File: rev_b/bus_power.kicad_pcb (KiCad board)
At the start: 2 copper layers, 50 x 50 mm, 18 parts, among them J1 TERMINATE_JUMPER, Q1 FQP47P06, Q2 FQP47P06, SW1 F-426-0020

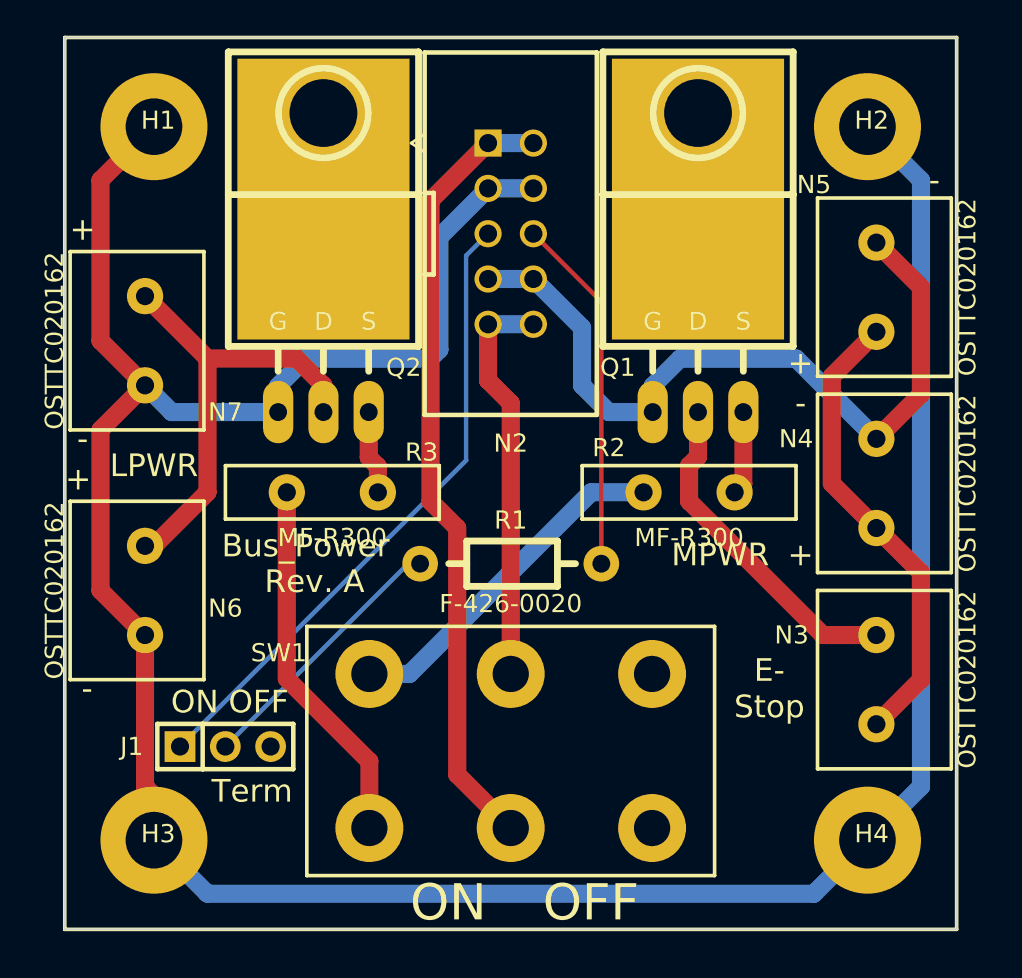
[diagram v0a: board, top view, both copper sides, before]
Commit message: Did first layout of Rev. B.
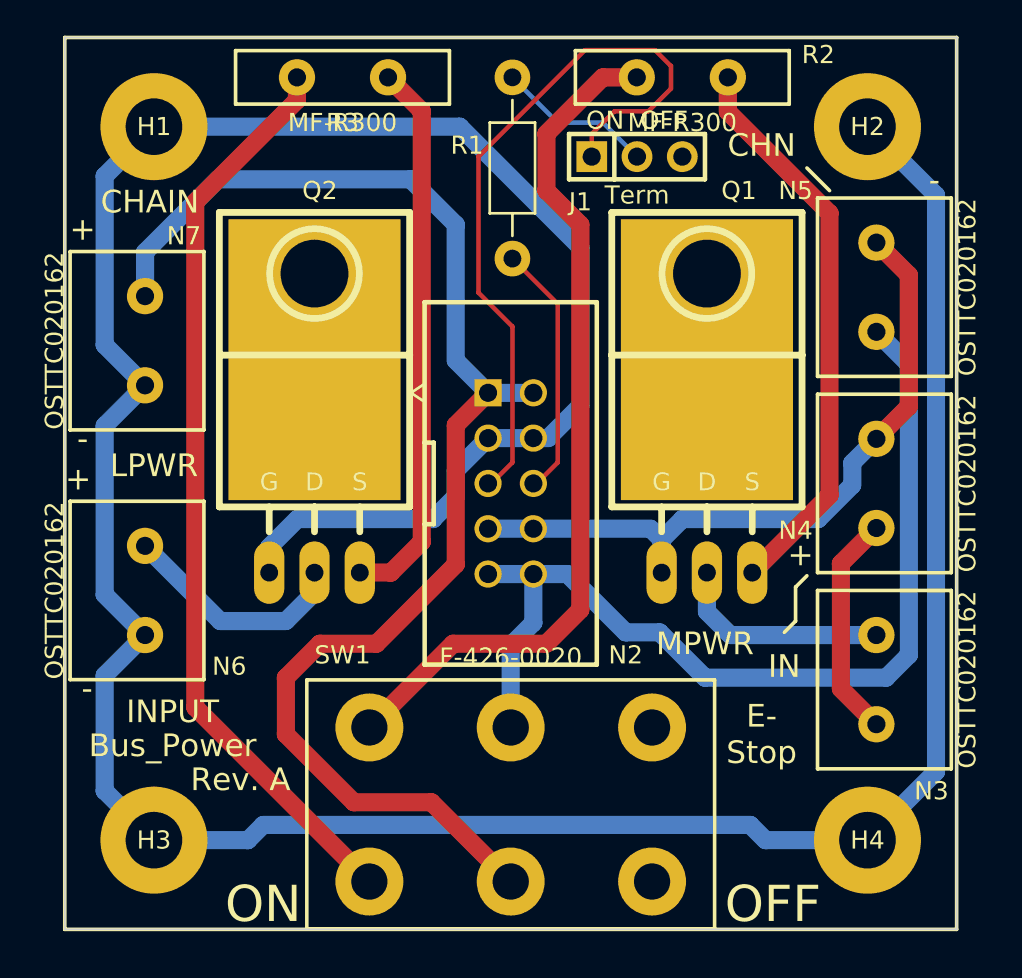
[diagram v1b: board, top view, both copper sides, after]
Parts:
- G1: footprint Bus_BeagleBone_Rev_A:OSHW_LOGO_400mil -> Bus_Power:OSHW_LOGO_400mil
- H1, H2, H3, H4: footprint Bus_BeagleBone_Rev_A:MountingHole_3mm -> Bus_Power:MountingHole_3mm
- J1: footprint Bus_BeagleBone_Rev_A:Pin_Header_Straight_1x03 -> Bus_Power:Pin_Header_Straight_1x03
- N2: footprint Bus_BeagleBone_Rev_A:Pin_Header_Straight_2x05_Shrouded -> Bus_Power:Pin_Header_Straight_2x05_Shrouded
- N3, N4, N5, N6, N7: footprint Bus_BeagleBone_Rev_A:5MM_TERMINAL_BLOCK_2_POS -> Bus_Power:5MM_TERMINAL_BLOCK_2_POS
- Q1, Q2: footprint Bus_BeagleBone_Rev_A:TO-220_FET-GDS_Horizontal_LargePads -> Bus_Power:TO-220_FET-GDS_Horizontal_LargePads
- R1: footprint Bus_BeagleBone_Rev_A:Resistor_Horizontal__400 -> Bus_Power:Resistor_Horizontal_400
- R2, R3: footprint Bus_Power_Rev_A:MF_R300 -> Bus_Power:MF_R300
- SW1: footprint Bus_Power_Rev_A:GF_426_0020 -> Bus_Power:GF_426_0020
- moved J1 40.3 mm to (132.1, 106.7)
- moved R3 23.3 mm to (115.6, 102.2)
- moved R2 23.3 mm to (134.6, 102.2)
- moved R1 22.2 mm to (125.1, 107.3), turned to 270 degrees
- moved N2 14.0 mm to (125.0, 125.0)
- moved G1 9.94 mm to (135.9, 120.0)
- moved Q1 9.01 mm to (136.0, 130.0)
- moved Q2 9.01 mm to (114.0, 130.0)
- moved SW1 3.00 mm to (125.0, 143.0)
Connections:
- net /BGND renamed /MGND
- net /BPWR2 renamed /MPWR1
- net /BPWR3 renamed /MPWR2
- net /BPWR4 renamed /MPWR3
- net /CANH renamed Net-(J1-Pad1)
- net /CANL renamed Net-(N2-Pad6)
- N2 pad 10: /BPWR5 -> /MPWR4
- N2 pad 9: /BPWR5 -> /MPWR4
- N3 pad 2: /BPWR1 -> /MPWR0
- N4 pad 2: /BPWR1 -> /MPWR0
- N5 pad 2: /BPWR1 -> /MPWR4
- N7 pad 2: /LPWR1 -> /LPWR4
- SW1 pad 2: /BPWR5 -> /MPWR4
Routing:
- net /MPWR4: track 0.00 -> 54.5 mm
- net /LPWR4: track 44.1 -> 77.1 mm
- net /LPWR3: track 20.7 -> 51.5 mm
- net /LGND: track 161.7 -> 191.0 mm
- net /MPWR3: track 19.6 -> 48.4 mm
- net /MPWR2: track 4.70 -> 31.9 mm
- net /LPWR2: track 4.71 -> 31.0 mm
- net /BPWR1: track 26.1 -> 0.00 mm
- net /BPWR5: track 22.7 -> 0.00 mm
- net /LPWR1: track 25.8 -> 13.0 mm
- net /MPWR0: track 0.00 -> 12.6 mm
- net /MPWR1: track 18.8 -> 12.2 mm
- net Net-(J1-Pad2): track 15.2 -> 8.83 mm
- net Net-(N2-Pad6): track 20.1 -> 14.3 mm
- net Net-(J1-Pad1): track 35.9 -> 41.5 mm
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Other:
- board text added: "Bus Power Rev. B 1Oct2014 (c) Gramlich"
- board text added: "CHAIN"
- board text added: "CHN"
- board text added: "IN"
- board text added: "INPUT"
- board text removed: "Bus Power Rev. A 11Aug2014 (c) Gramlich"
